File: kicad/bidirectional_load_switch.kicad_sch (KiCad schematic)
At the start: 9 parts, among them J101 Screw_Terminal_01x13

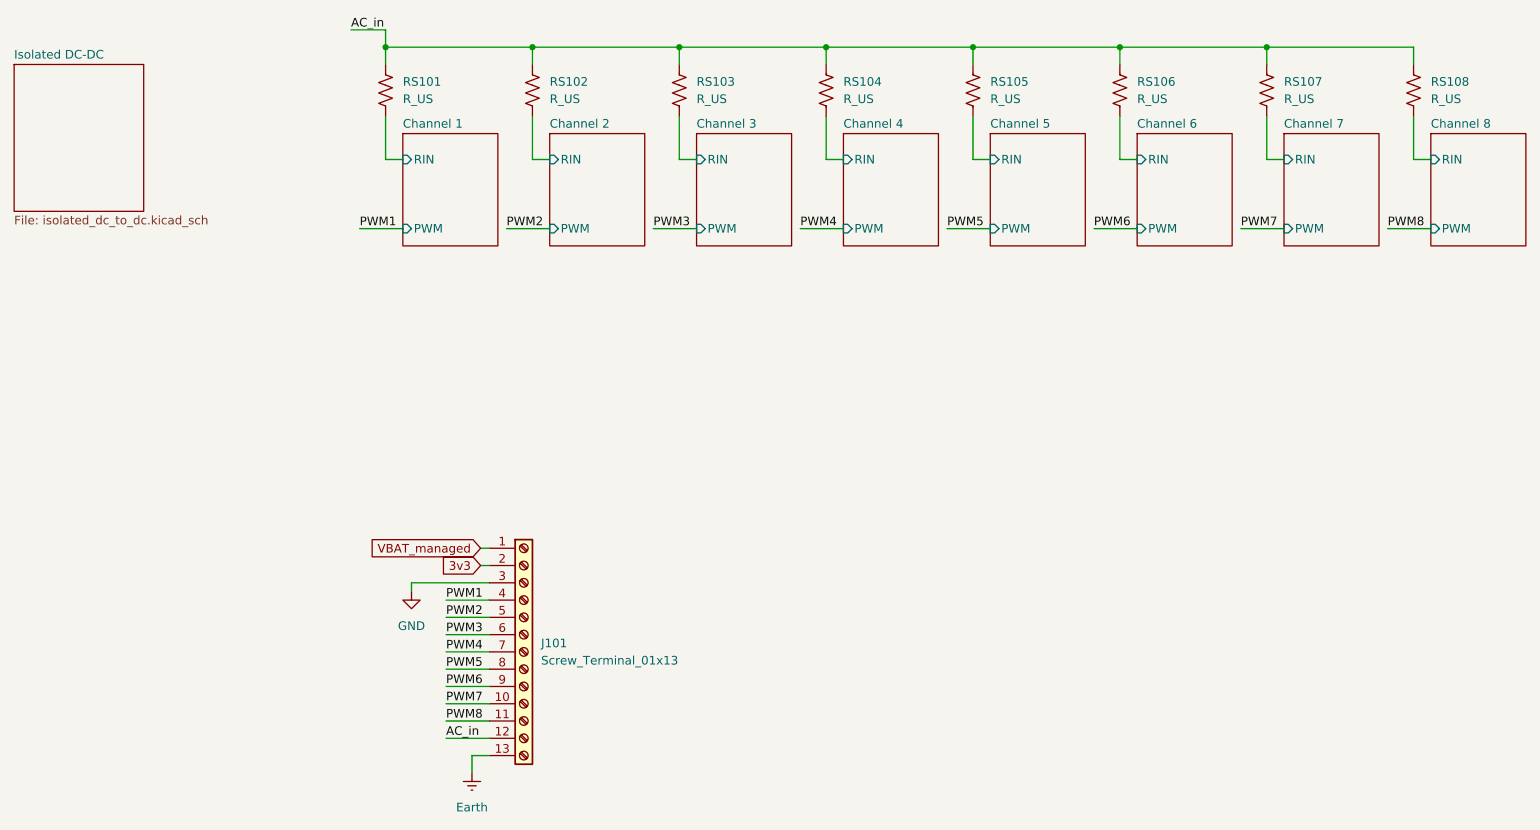
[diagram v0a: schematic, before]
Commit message: kicad
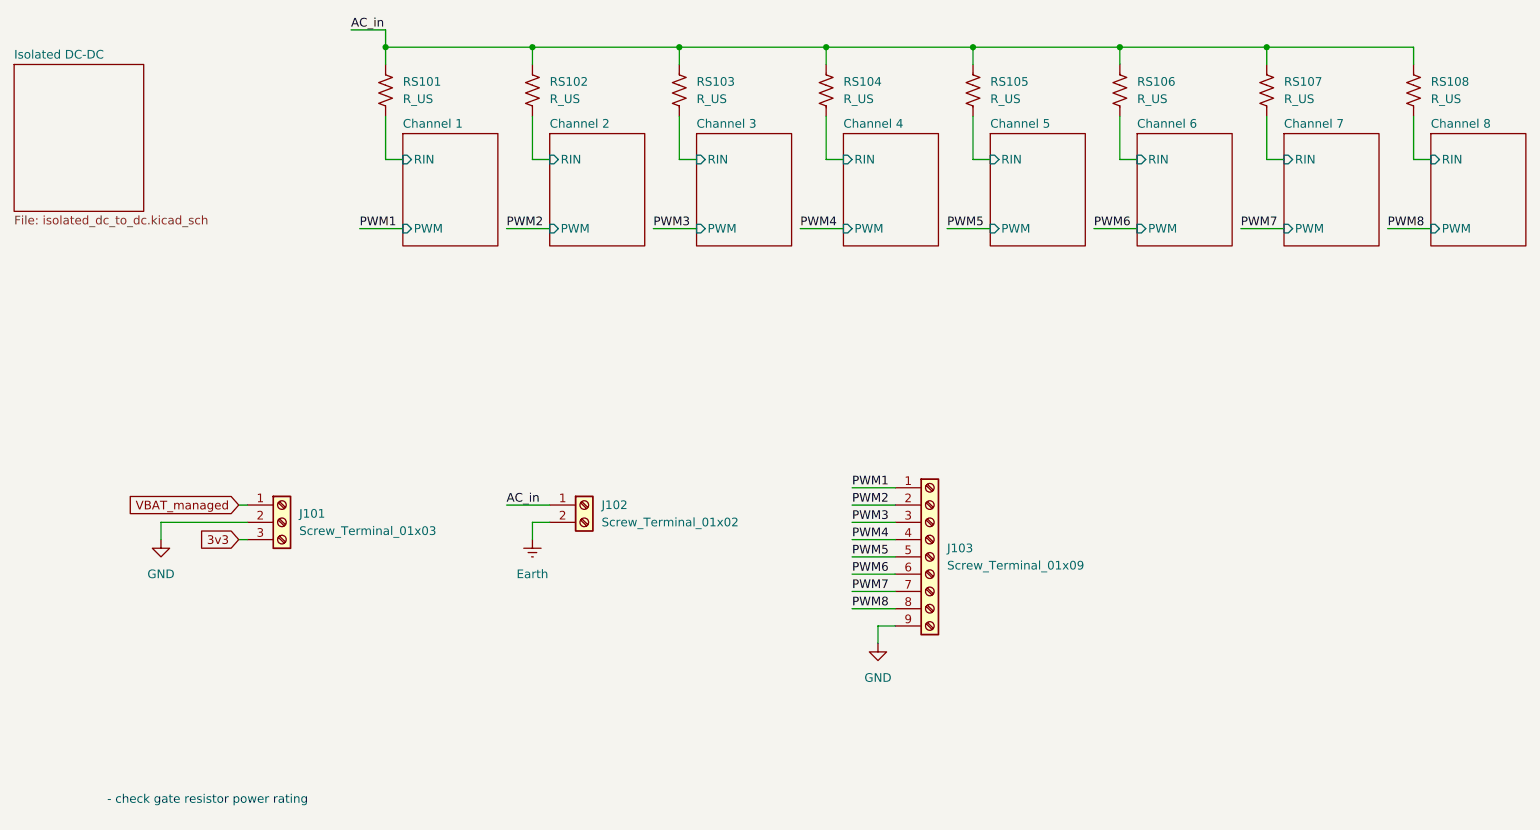
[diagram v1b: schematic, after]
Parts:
- removed J101: Screw_Terminal_01x13, TerminalBlock:TerminalBlock_Xinya_XY308-2.54-13P_1x13_P2.54mm_Horizontal, symbol Connector:Screw_Terminal_01x13
- added J101: Screw_Terminal_01x03, TerminalBlock:TerminalBlock_Xinya_XY308-2.54-3P_1x03_P2.54mm_Horizontal, symbol Connector:Screw_Terminal_01x03
- added J102: Screw_Terminal_01x02, TerminalBlock:TerminalBlock_Xinya_XY308-2.54-2P_1x02_P2.54mm_Horizontal, symbol Connector:Screw_Terminal_01x02
- added J103: Screw_Terminal_01x09, TerminalBlock:TerminalBlock_Xinya_XY308-2.54-9P_1x09_P2.54mm_Horizontal, symbol Connector:Screw_Terminal_01x09
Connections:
- net 3v3: now also J101.3 (Pin_3)
- net AC_in: now also J102.1 (Pin_1)
- net Earth: now also J102.2 (Pin_2)
- net GND: now also J101.2 (Pin_2), J103.9 (Pin_9)
- net PWM1: now also J103.1 (Pin_1)
- net PWM2: now also J103.2 (Pin_2)
- net PWM3: now also J103.3 (Pin_3)
- net PWM4: now also J103.4 (Pin_4)
- net PWM5: now also J103.5 (Pin_5)
- net PWM6: now also J103.6 (Pin_6)
- net PWM7: now also J103.7 (Pin_7)
- net PWM8: now also J103.8 (Pin_8)
- net VBAT_managed: now also J101.1 (Pin_1)
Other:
- note added: "- check gate resistor power rating"

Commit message: kicad
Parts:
- RS101, RS102, RS103, RS104, RS105, RS106, RS107, RS108: footprint Resistor_SMD:R_1206_3216Metric_Pad1.30x1.75mm_HandSolder -> Resistor_SMD:R_2512_6332Metric
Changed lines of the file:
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@@
 			)
 		)
-		(property "Footprint" "Resistor_SMD:R_1206_3216Metric_Pad1.30x1.75mm_HandSolder"
+		(property "Footprint" "Resistor_SMD:R_2512_6332Metric"
 			(at 126.746 35.814 90)
 			(effects
@@
 			)
 		)
-		(property "Footprint" "Resistor_SMD:R_1206_3216Metric_Pad1.30x1.75mm_HandSolder"
+		(property "Footprint" "Resistor_SMD:R_2512_6332Metric"
 			(at 234.696 35.814 90)
 			(effects
@@
 			)
 		)
-		(property "Footprint" "Resistor_SMD:R_1206_3216Metric_Pad1.30x1.75mm_HandSolder"
+		(property "Footprint" "Resistor_SMD:R_2512_6332Metric"
 			(at 105.156 35.814 90)
 			(effects
@@
 			)
 		)
-		(property "Footprint" "Resistor_SMD:R_1206_3216Metric_Pad1.30x1.75mm_HandSolder"
+		(property "Footprint" "Resistor_SMD:R_2512_6332Metric"
 			(at 169.926 35.814 90)
 			(effects
@@
 			)
 		)
-		(property "Footprint" "Resistor_SMD:R_1206_3216Metric_Pad1.30x1.75mm_HandSolder"
+		(property "Footprint" "Resistor_SMD:R_2512_6332Metric"
 			(at 191.516 35.814 90)
 			(effects
@@
 			)
 		)
-		(property "Footprint" "Resistor_SMD:R_1206_3216Metric_Pad1.30x1.75mm_HandSolder"
+		(property "Footprint" "Resistor_SMD:R_2512_6332Metric"
 			(at 213.106 35.814 90)
 			(effects
@@
 			)
 		)
-		(property "Footprint" "Resistor_SMD:R_1206_3216Metric_Pad1.30x1.75mm_HandSolder"
+		(property "Footprint" "Resistor_SMD:R_2512_6332Metric"
 			(at 148.336 35.814 90)
 			(effects
@@
 			)
 		)
-		(property "Footprint" "Resistor_SMD:R_1206_3216Metric_Pad1.30x1.75mm_HandSolder"
+		(property "Footprint" "Resistor_SMD:R_2512_6332Metric"
 			(at 83.566 35.814 90)
 			(effects
